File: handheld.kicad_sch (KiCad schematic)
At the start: 19 parts, among them J1 Conn_01x15_Pin, J2 Conn_01x15_Pin, J3 Conn_02x13_Odd_Even, J6 Micro_SD_Card, SW1 SW_Push, SW10 SW_Push, SW11 SW_Push, SW12 SW_Push, SW2 SW_Push, SW3 SW_Push, SW4 SW_Push, SW5 SW_Push, SW6 SW_Push, SW7 SW_Push, SW8 SW_Push, SW9 SW_Push, U1 MCP23017x-x-SP

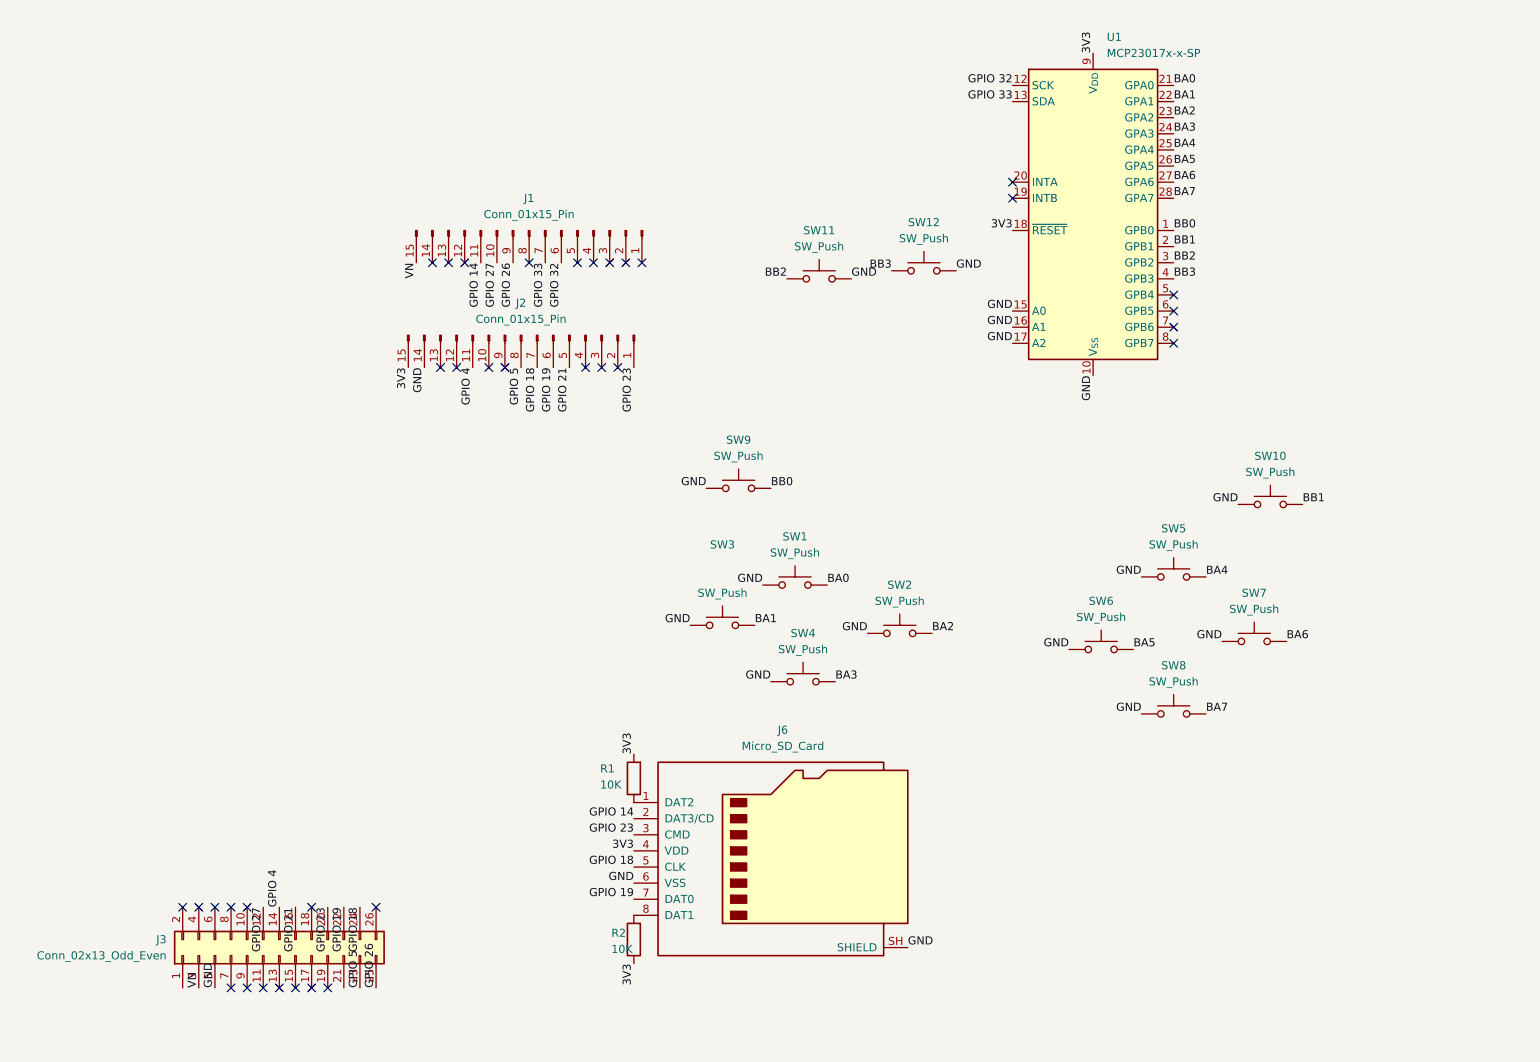
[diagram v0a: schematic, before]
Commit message: final pcb and schematic
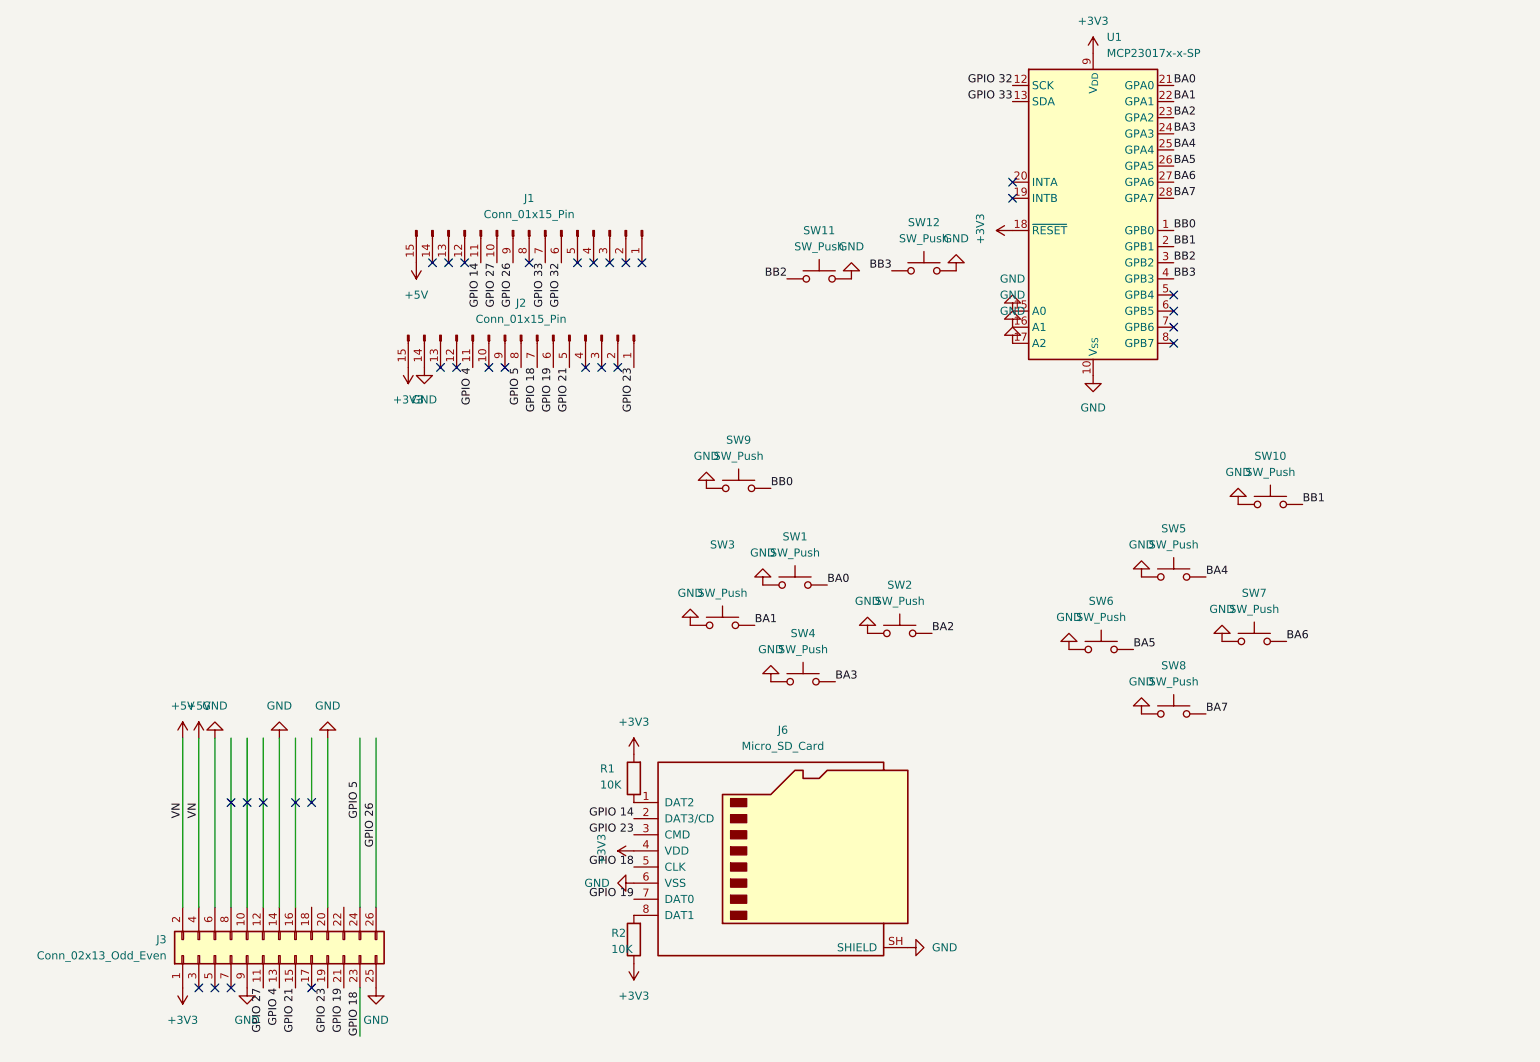
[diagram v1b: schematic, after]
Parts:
- J3: footprint Connector_PinSocket_2.54mm:PinSocket_2x13_P2.54mm_Vertical -> Connector_PinHeader_2.54mm:PinHeader_2x13_P2.54mm_Vertical
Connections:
- net 3V3 is gone; now on net +3V3: J2.15 (Pin_15), J6.4 (VDD), R1.2, R2.1, U1.18 (~{RESET}), U1.9 (V_{DD})
- net GND: now also J3.14 (Pin_14), J3.20 (Pin_20), J3.25 (Pin_25), J3.6 (Pin_6), J3.9 (Pin_9); no longer J3.5 (Pin_5)
- net GPIO 18: now also J3.23 (Pin_23); no longer J3.24 (Pin_24)
- net GPIO 19: now also J3.21 (Pin_21); no longer J3.22 (Pin_22)
- net GPIO 21: now also J3.15 (Pin_15); no longer J3.16 (Pin_16)
- net GPIO 23: now also J3.19 (Pin_19); no longer J3.20 (Pin_20)
- net GPIO 26: now also J3.26 (Pin_26); no longer J3.25 (Pin_25)
- net GPIO 27: now also J3.11 (Pin_11); no longer J3.12 (Pin_12)
- net GPIO 4: now also J3.13 (Pin_13); no longer J3.14 (Pin_14)
- net GPIO 5: now also J3.24 (Pin_24); no longer J3.23 (Pin_23)
- net +3V3: now reaches J3.1 (Pin_1)
- net +5V: now reaches J3.2 (Pin_2)
- net +5V: now also J1.15 (Pin_15), J3.4 (Pin_4)
- net VN: no longer names the net of J3.3 (Pin_3)
- net VN: no longer J1.15 (Pin_15)
- no-connect marks 36 -> 31

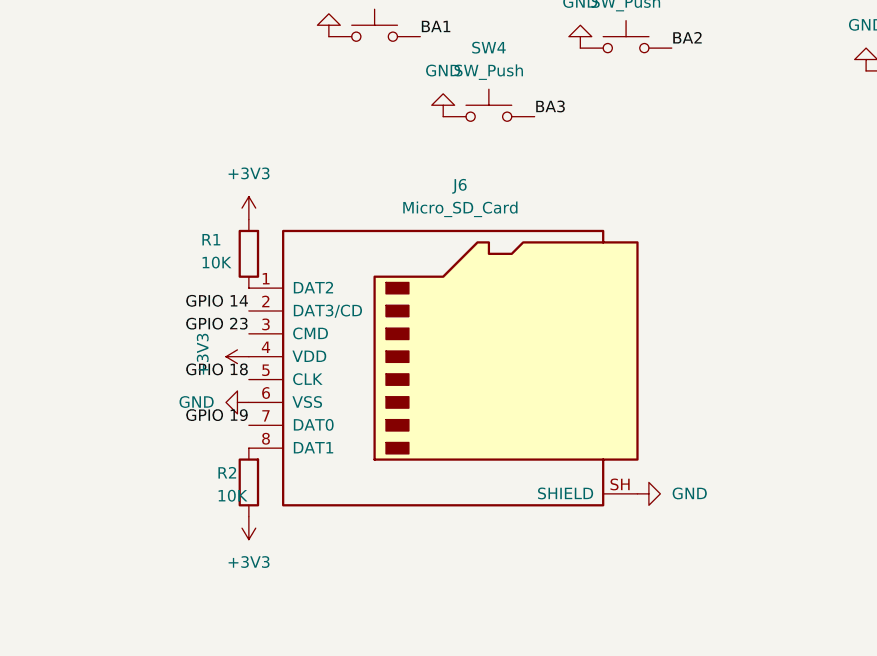
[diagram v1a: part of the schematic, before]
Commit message: final pcb
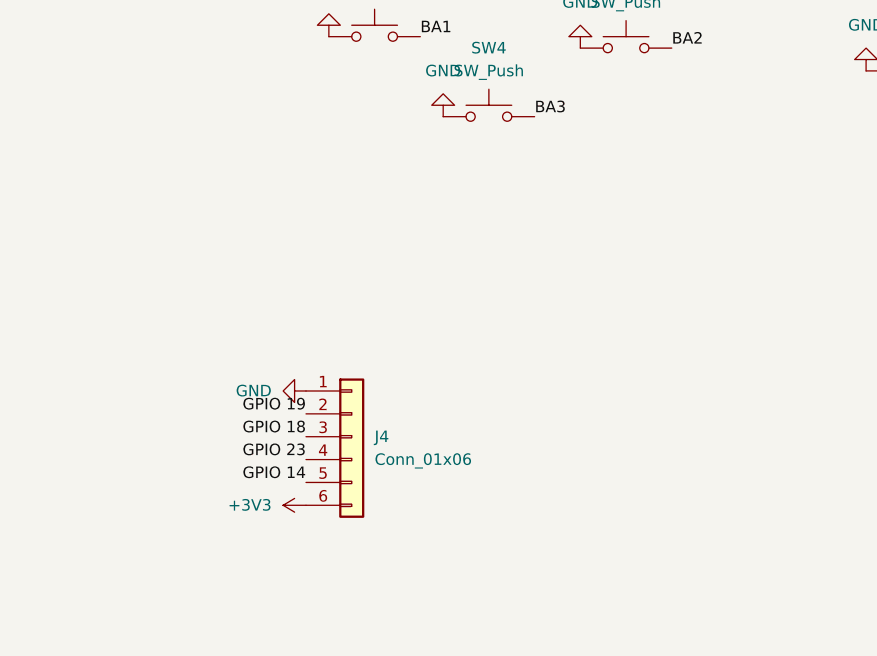
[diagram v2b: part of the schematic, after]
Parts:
- removed J6: Micro_SD_Card, Connector_Card:microSD_HC_Wuerth_693072010801, symbol Connector:Micro_SD_Card
- removed R1, R2: 10K, Resistor_SMD:R_0805_2012Metric, symbol Device:R
- added J4: Conn_01x06, Connector_PinHeader_2.54mm:PinHeader_1x06_P2.54mm_Vertical, symbol Connector_Generic:Conn_01x06
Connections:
- net +3V3: now also J4.6 (Pin_6)
- net GND: now also J4.1 (Pin_1)
- net GPIO 14: now also J4.5 (Pin_5)
- net GPIO 18: now also J4.3 (Pin_3)
- net GPIO 19: now also J4.2 (Pin_2)
- net GPIO 23: now also J4.4 (Pin_4)

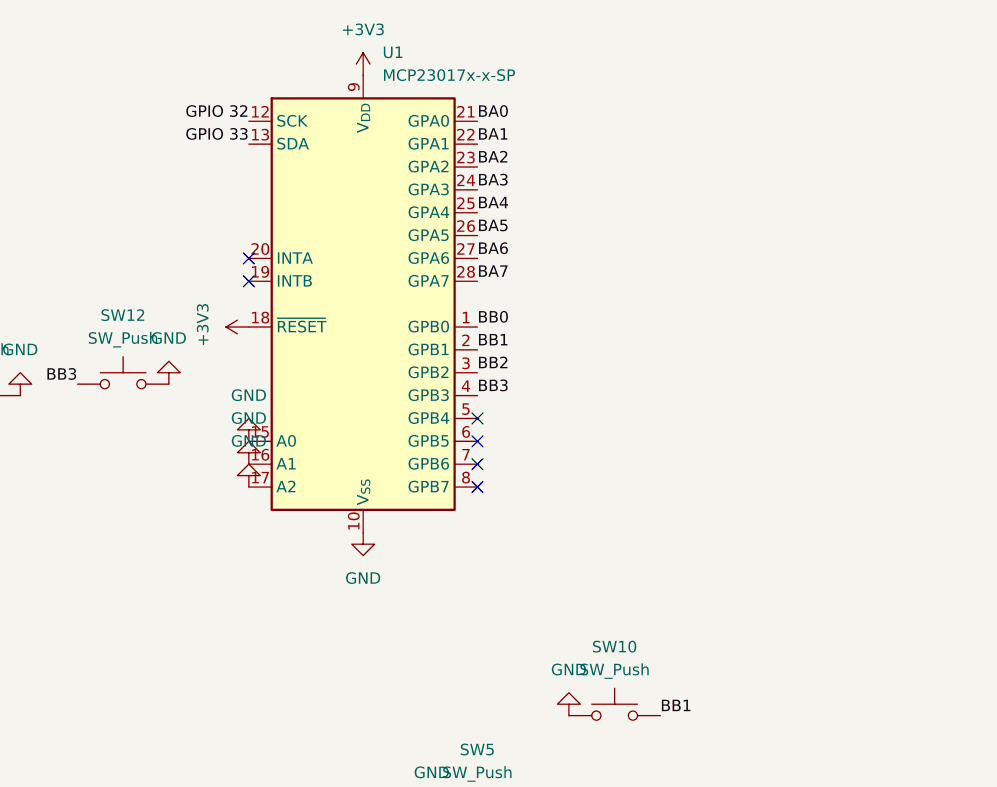
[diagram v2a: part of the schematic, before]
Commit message: final pcb
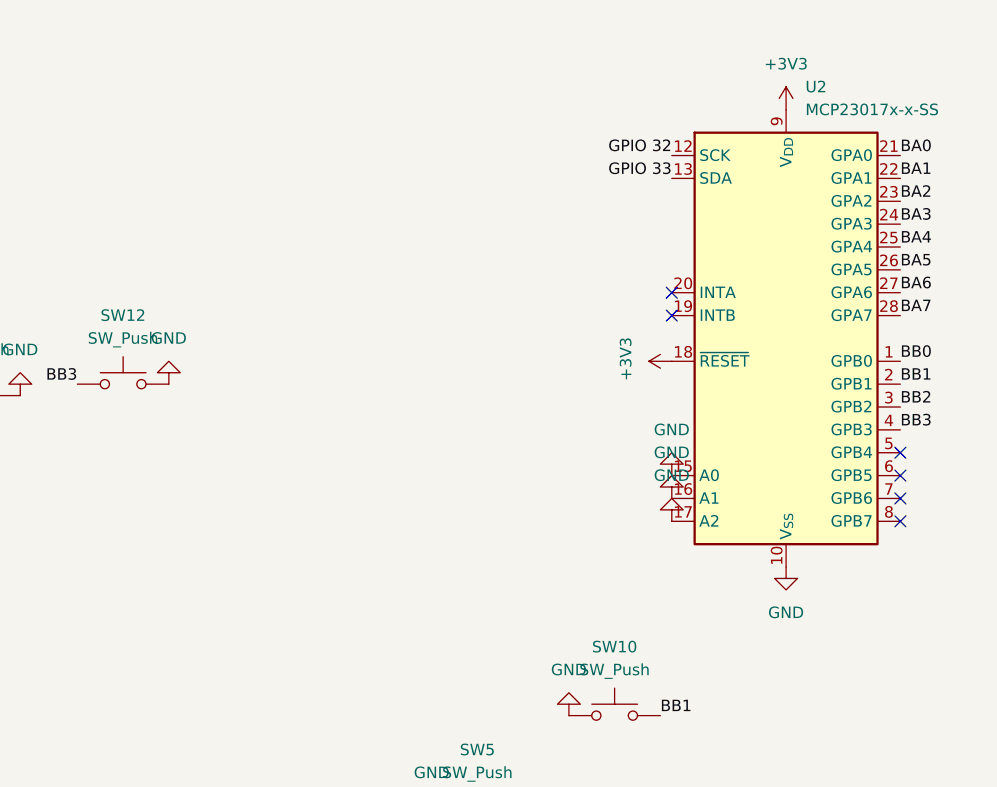
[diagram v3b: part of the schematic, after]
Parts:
- removed U1: MCP23017x-x-SP, Package_DIP:DIP-28_W7.62mm, symbol Interface_Expansion:MCP23017x-x-SP
- added U2: MCP23017x-x-SS, Package_SO:SSOP-28_5.3x10.2mm_P0.65mm, symbol Interface_Expansion:MCP23017x-x-SS
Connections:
- net +3V3: now also U2.18 (~{RESET}), U2.9 (V_{DD})
- net BA0: now also U2.21 (GPA0)
- net BA1: now also U2.22 (GPA1)
- net BA2: now also U2.23 (GPA2)
- net BA3: now also U2.24 (GPA3)
- net BA4: now also U2.25 (GPA4)
- net BA5: now also U2.26 (GPA5)
- net BA6: now also U2.27 (GPA6)
- net BA7: now also U2.28 (GPA7)
- net BB0: now also U2.1 (GPB0)
- net BB1: now also U2.2 (GPB1)
- net BB2: now also U2.3 (GPB2)
- net BB3: now also U2.4 (GPB3)
- net GND: now also U2.10 (V_{SS}), U2.15 (A0), U2.16 (A1), U2.17 (A2)
- net GPIO 32: now also U2.12 (SCK)
- net GPIO 33: now also U2.13 (SDA)
